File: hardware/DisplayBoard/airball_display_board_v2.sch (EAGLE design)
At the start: 51 parts, among them J2 105450-0101, J4 105450-0101, J5 SCREW_TERMINAL_8POS, J6 SCREW_TERMINAL_8POS, SW1 TL1014BF160QG, SW2 TL1014BF160QG, SW3 TL1014BF160QG, SW4 TL1014BF160QG, SW5 TL1014BF160QG, U10 DS3231, U2 TFP401A, U3 TFT_40PIN_FFC-BOT, U5 TPS61169

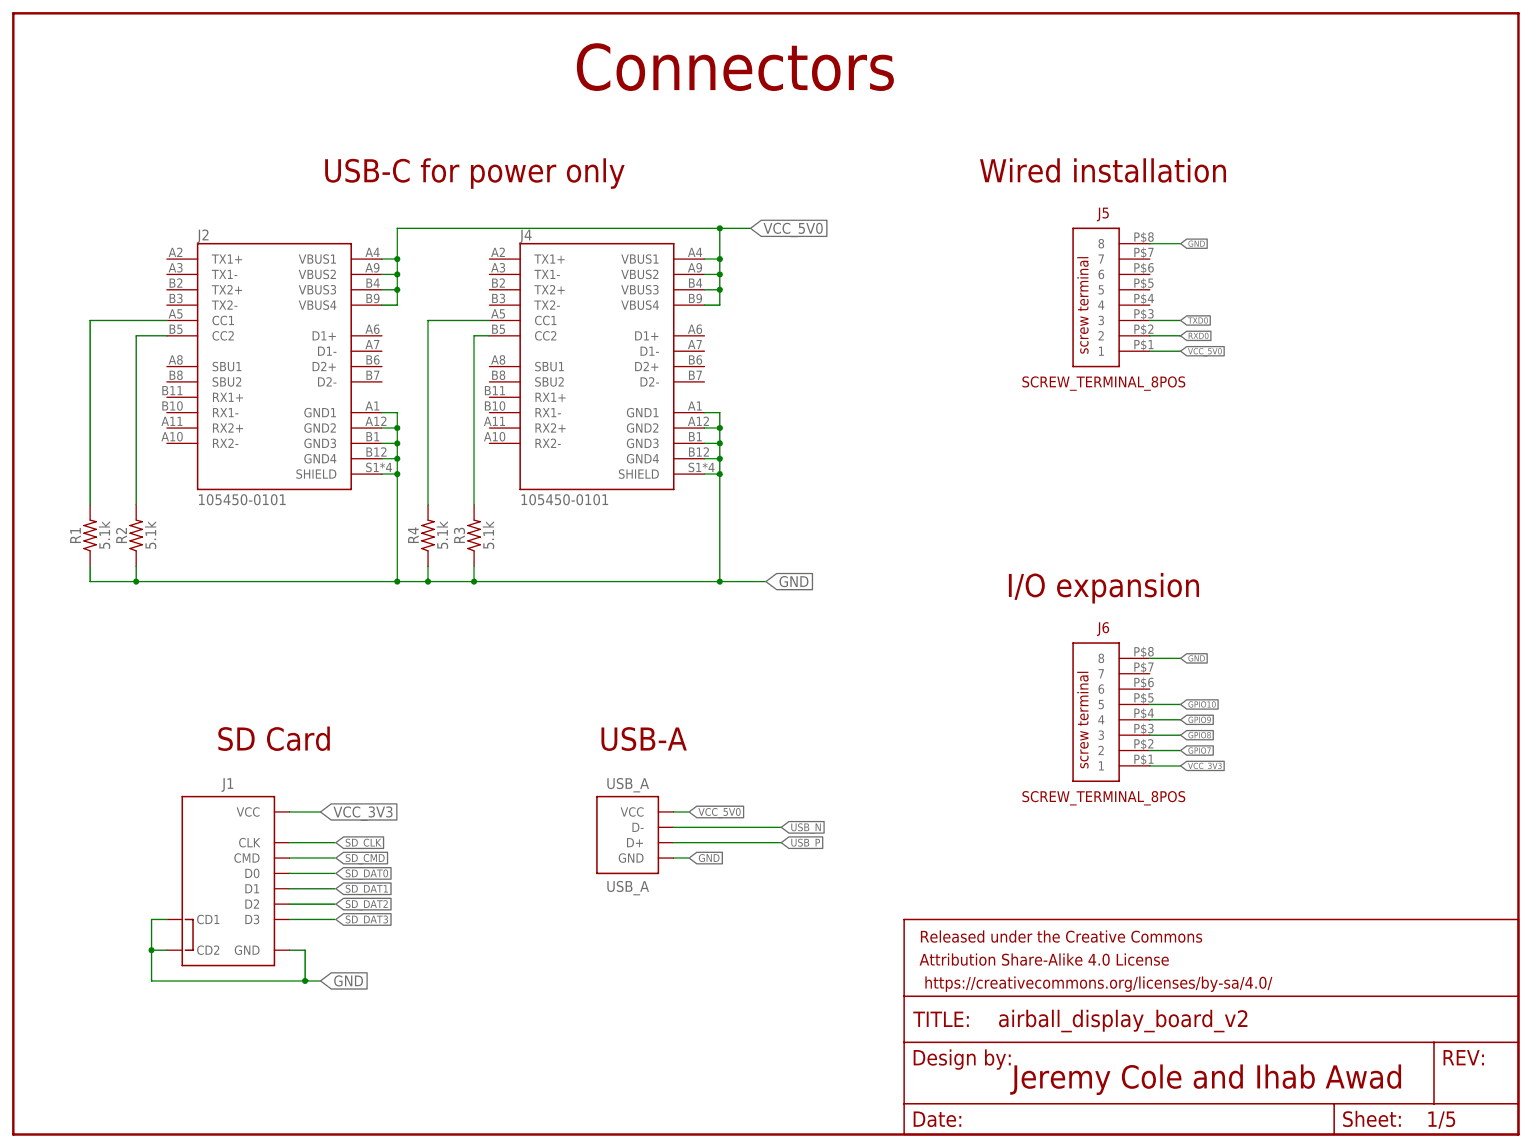
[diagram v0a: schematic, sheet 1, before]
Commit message: Minor improvements to display board.
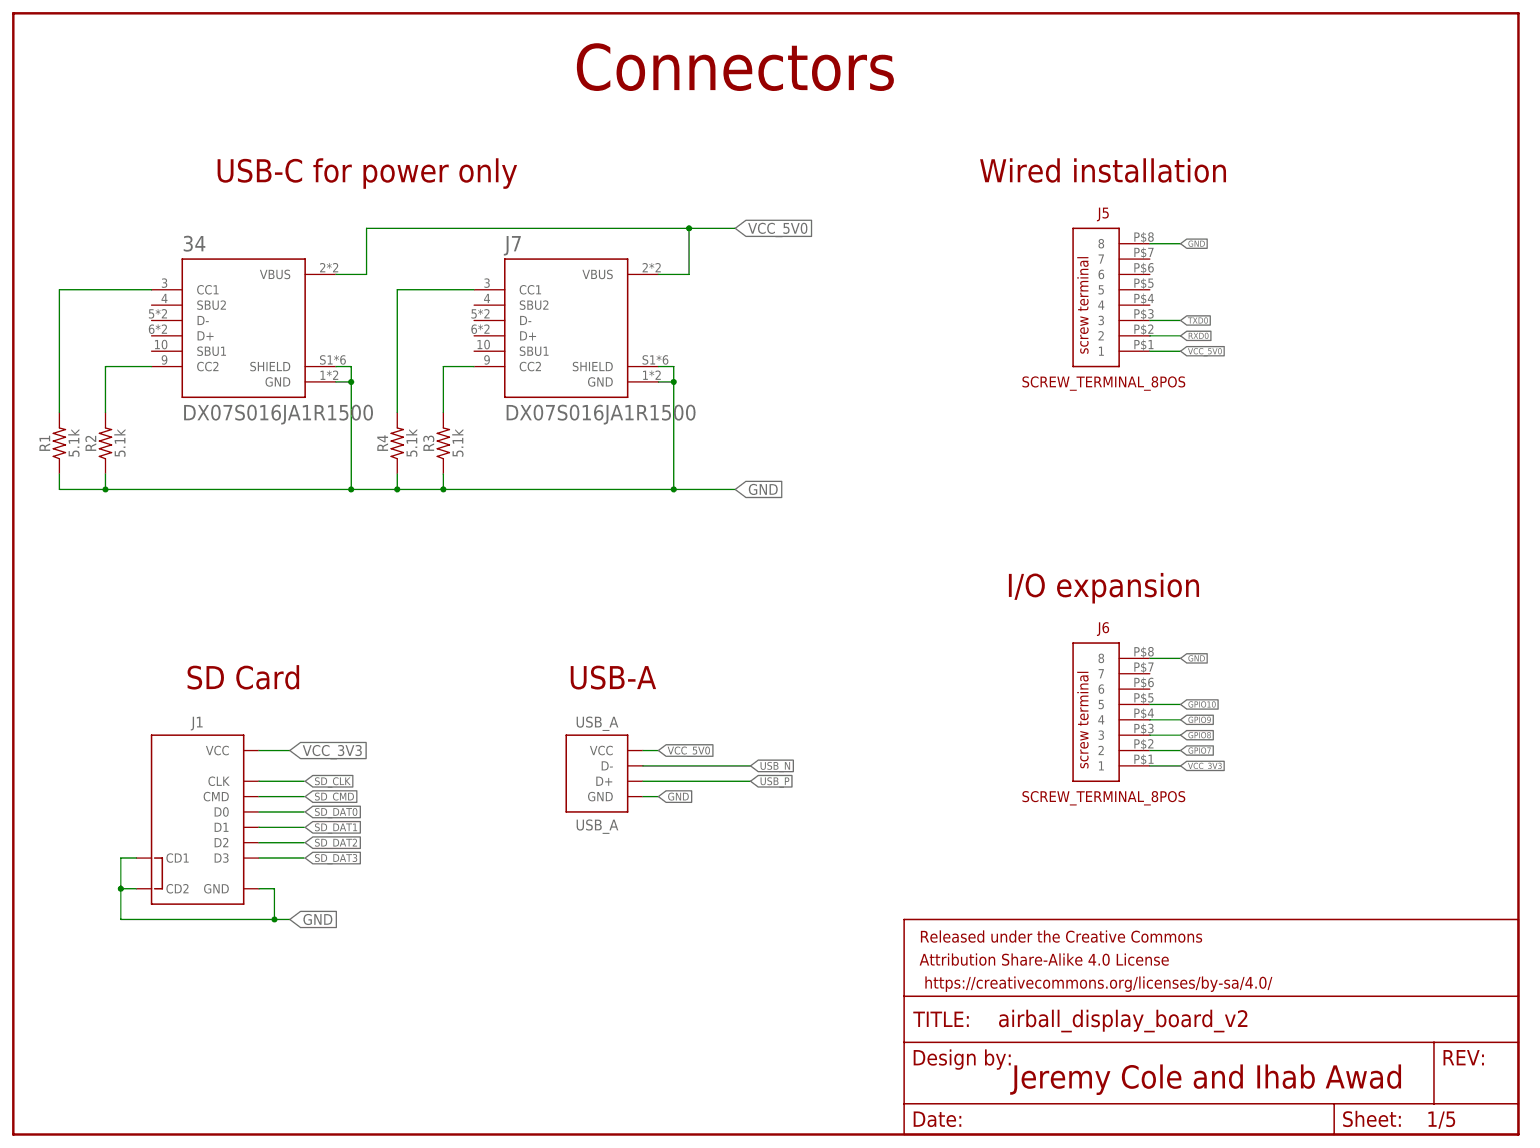
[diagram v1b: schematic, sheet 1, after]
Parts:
- removed J2, J4: 105450-0101, 105450-0101:105450-0101
- added 34, J7: DX07S016JA1R1500, airball:DX07S016JA1R1500
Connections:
- net GND: now also 34.GND, 34.SHIELD, J7.GND, J7.SHIELD; no longer J2.GND1, J2.GND2, J2.GND3, J2.GND4, J2.SHIELD, J4.GND1, J4.GND2, J4.GND3, J4.GND4, J4.SHIELD
- net N$1: now also 34.CC2; no longer J2.CC2
- net N$2: now also 34.CC1; no longer J2.CC1
- net N$3: now also J7.CC2; no longer J4.CC2
- net N$4: now also J7.CC1; no longer J4.CC1
- net VCC_5V0: now also 34.VBUS, J7.VBUS; no longer J2.VBUS1, J2.VBUS2, J2.VBUS3, J2.VBUS4, J4.VBUS1, J4.VBUS2, J4.VBUS3, J4.VBUS4
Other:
- moved on the sheet: J1, R1, R2, R3, R4, USB_A
